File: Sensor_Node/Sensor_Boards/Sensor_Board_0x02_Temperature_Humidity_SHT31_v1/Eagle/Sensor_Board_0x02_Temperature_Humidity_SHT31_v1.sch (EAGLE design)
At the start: 15 parts, among them J1 M04_SMD_90, J2 M07_SMD_STRAIGHT, J4 ARDUINO_ISP, U2 ATMEGA328P_TQFP, Y1 8MHZ

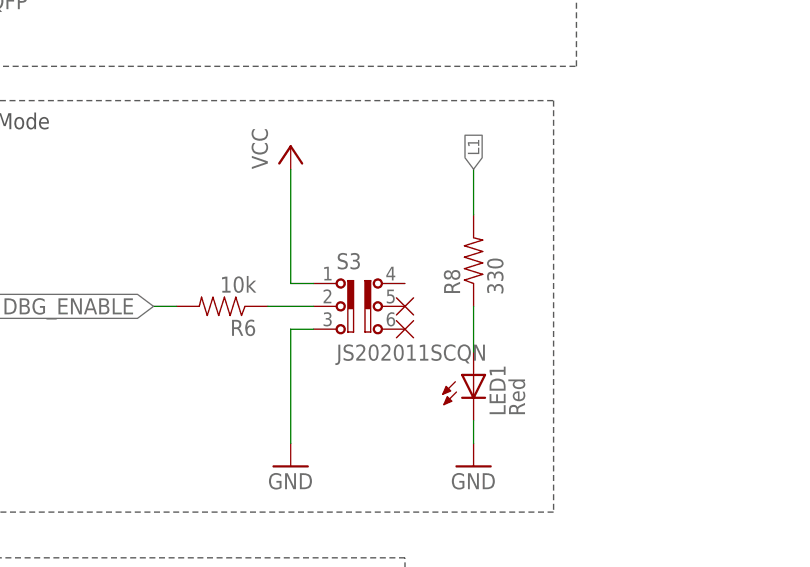
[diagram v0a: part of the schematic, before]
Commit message: Revert "Changed something"
This reverts commit e7fad535a0aed3b7ca3650d1b08948d39ff050b6.
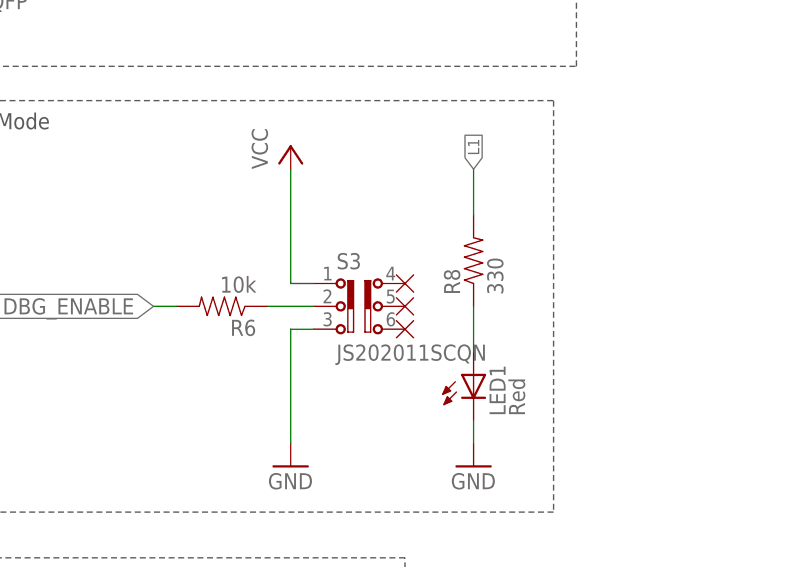
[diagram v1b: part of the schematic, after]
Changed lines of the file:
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@@
 <?xml version="1.0" encoding="utf-8"?>
 <!DOCTYPE eagle SYSTEM "eagle.dtd">
-<eagle version="8.1.0">
+<eagle version="8.1.1">
 <drawing>
 <settings>
@@
 <part name="U$12" library="myownthings" deviceset="N/C" device=""/>
 <part name="U$13" library="myownthings" deviceset="N/C" device=""/>
+<part name="U$14" library="myownthings" deviceset="N/C" device=""/>
 <part name="U$15" library="myownthings" deviceset="N/C" device=""/>
 <part name="U$16" library="myownthings" deviceset="N/C" device=""/>
@@
 <instance part="U$12" gate="G$1" x="86.36" y="139.7"/>
 <instance part="U$13" gate="G$1" x="86.36" y="137.16"/>
+<instance part="U$14" gate="G$1" x="106.68" y="93.98"/>
 <instance part="U$15" gate="G$1" x="106.68" y="91.44"/>
 <instance part="U$16" gate="G$1" x="106.68" y="88.9"/>

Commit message: Changed something
yes
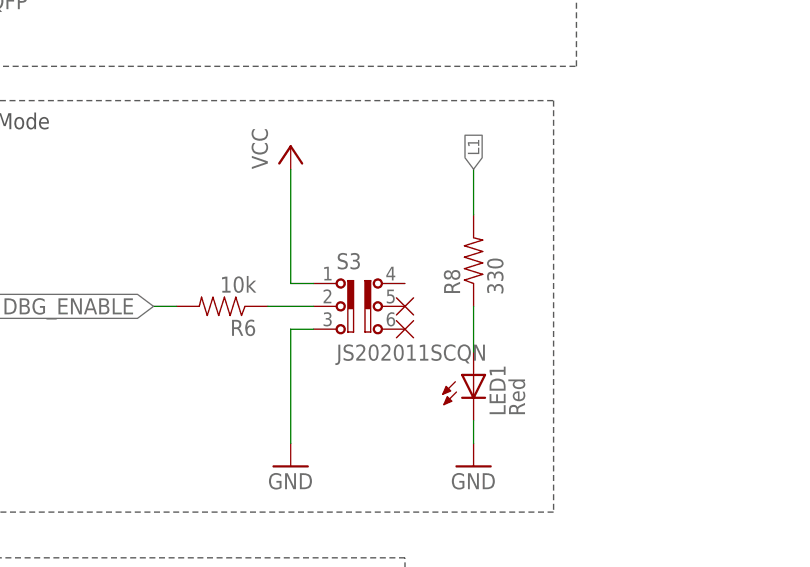
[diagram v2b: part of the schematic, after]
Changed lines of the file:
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@@
 <?xml version="1.0" encoding="utf-8"?>
 <!DOCTYPE eagle SYSTEM "eagle.dtd">
-<eagle version="8.1.1">
+<eagle version="8.1.0">
 <drawing>
 <settings>
@@
 <part name="U$12" library="myownthings" deviceset="N/C" device=""/>
 <part name="U$13" library="myownthings" deviceset="N/C" device=""/>
-<part name="U$14" library="myownthings" deviceset="N/C" device=""/>
 <part name="U$15" library="myownthings" deviceset="N/C" device=""/>
 <part name="U$16" library="myownthings" deviceset="N/C" device=""/>
@@
 <instance part="U$12" gate="G$1" x="86.36" y="139.7"/>
 <instance part="U$13" gate="G$1" x="86.36" y="137.16"/>
-<instance part="U$14" gate="G$1" x="106.68" y="93.98"/>
 <instance part="U$15" gate="G$1" x="106.68" y="91.44"/>
 <instance part="U$16" gate="G$1" x="106.68" y="88.9"/>
